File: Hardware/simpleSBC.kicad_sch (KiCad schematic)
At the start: 65 parts, among them J1 Conn_02x07_Odd_Even, J5 USB_A, J6 USB_A, J7 RJ45_Wuerth_7499010121A, J9 Conn_01x06, SW1 SW_Push, U1 STM32MP157FAD1, U2 STMPS2252MTR, U5 USBLC6-4SC6, U6 LAN8742A, X1 ASCO, Y1 32.786, Y2 X53T-C20SSA-25.000MHz

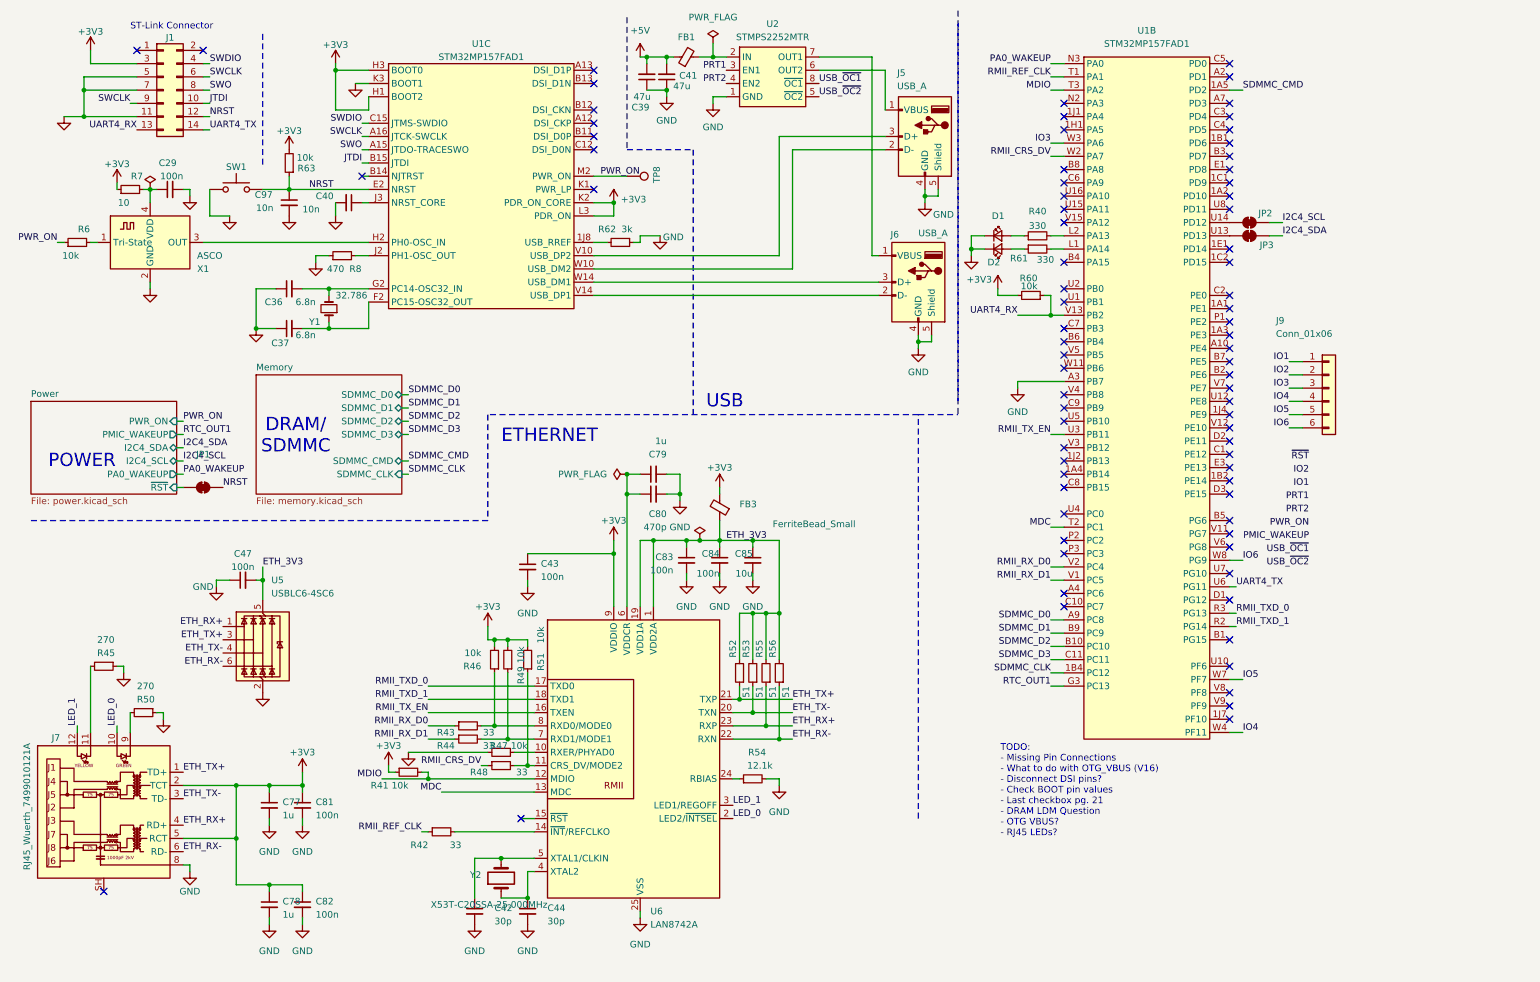
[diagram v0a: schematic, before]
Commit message: First Pass Routing
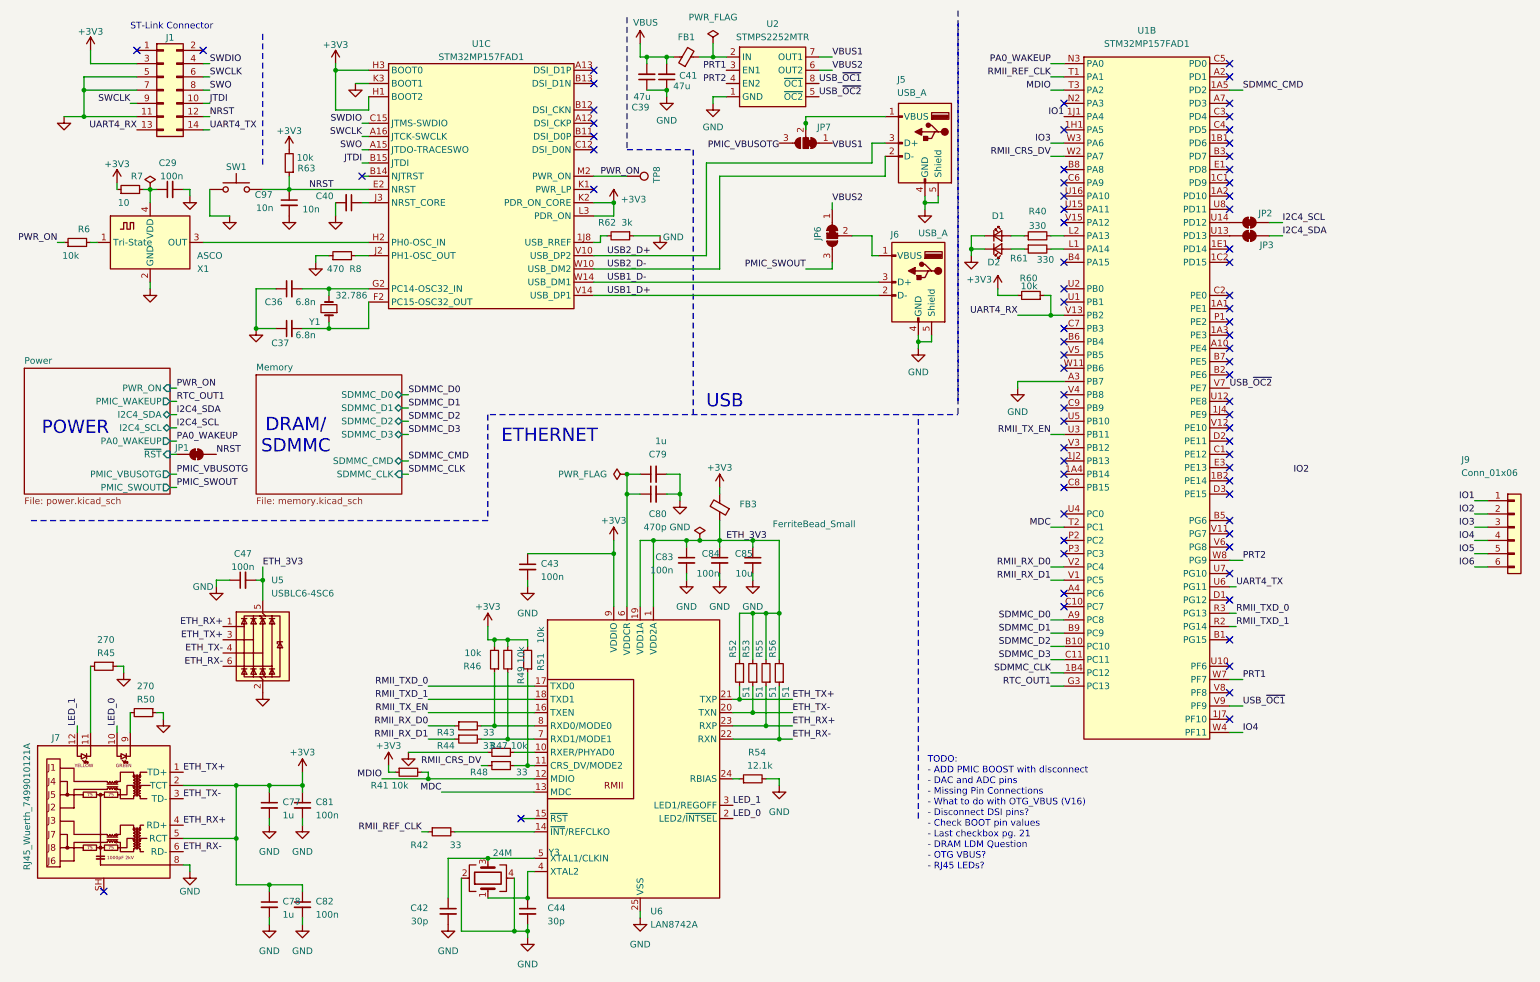
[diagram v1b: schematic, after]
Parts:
- removed Y2: X53T-C20SSA-25.000MHz, symbol Device:Crystal
- added JP6, JP7: SolderJumper_3_Bridged12, Jumper:SolderJumper-3_P1.3mm_Bridged2Bar12_Pad1.0x1.5mm, symbol Jumper:SolderJumper_3_Bridged12
- added Y3: 24M, SimpleSBC:Crystal_2.00x1.60mm, symbol Device:Crystal_GND24
- JP1, JP2, JP3: footprint (none) -> Resistor_SMD:R_0402_1005Metric; now in the parts list
- SW1: footprint (none) -> Button_Switch_SMD:SW_SPST_Omron_B3FS-101xP
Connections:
- net GND: now also Y3.2, Y3.4
- net IO1: now also U1.1J1 (PA4)
- net IO5: no longer U1.W7 (PF7)
- net IO6: no longer U1.W8 (PG9)
- net PRT1: now also U1.W7 (PF7)
- net PRT2: now also U1.W8 (PG9)
- net USB_~{OC1}: now also U1.V9 (PF9)
- net USB_~{OC2}: now also U1.V7 (PE7)
- net at J5.1 (VBUS): now also JP7.2 (C); no longer U2.6 (OUT2)
- net USB2_D-: now reaches J5.2 (D-), U1.W10 (USB_DM2)
- net USB2_D+: now reaches J5.3 (D+), U1.V10 (USB_DP2)
- net at J6.1 (VBUS): now also JP6.2 (C); no longer U2.7 (OUT1)
- net USB1_D+: now reaches J6.2 (D-), U1.V14 (USB_DP1)
- net USB1_D-: now reaches J6.3 (D+), U1.W14 (USB_DM1)
- net at C44.1, U6.4 (XTAL2): now also Y3.1
- net at C42.1, U6.5 (XTAL1/CLKIN): now also Y3.3
- net +5V renamed VBUS
- new net PMIC_SWOUT: JP6.3 (B)
- new net VBUS1: U2.7 (OUT1)
- new net VBUS2: JP6.1 (A), U2.6 (OUT2)
- no-connect marks 78 -> 75
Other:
- sheet Power ports: added PMIC_SWOUT, PMIC_VBUSOTG; removed none
- note added: "TODO: - ADD PMIC BOOST with disconnect - DAC and ADC pins - Missing Pin Connections - What to do with OTG_VBUS (V16) - Disconnect DSI pins? - Check BOOT pin values - Last checkbox pg. 21 - DRAM LDM Question - OTG VBUS? - RJ45 LEDs?"
- note removed: "TODO: - Missing Pin Connections - What to do with OTG_VBUS (V16) - Disconnect DSI pins? - Check BOOT pin values - Last checkbox pg. 21 - DRAM LDM Question - OTG VBUS? - RJ45 LEDs?"
- moved on the sheet: C42, J5, J9, JP1, R62
